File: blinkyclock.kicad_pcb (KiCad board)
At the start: 2 copper layers, 14 parts, among them J1 USB_OTG, J2 RTC, SW1 SW_Push, U1 ATTINY85-20PU

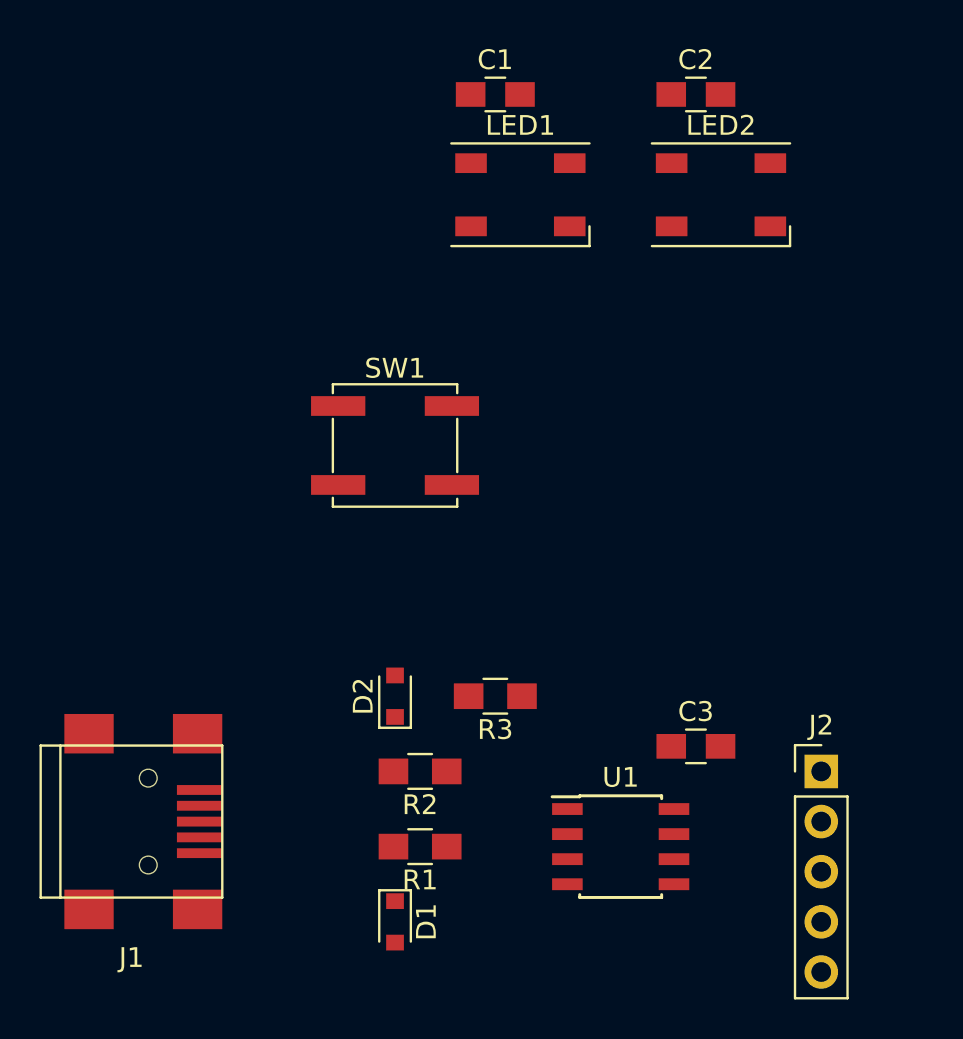
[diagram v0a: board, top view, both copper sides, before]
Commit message: finished layout
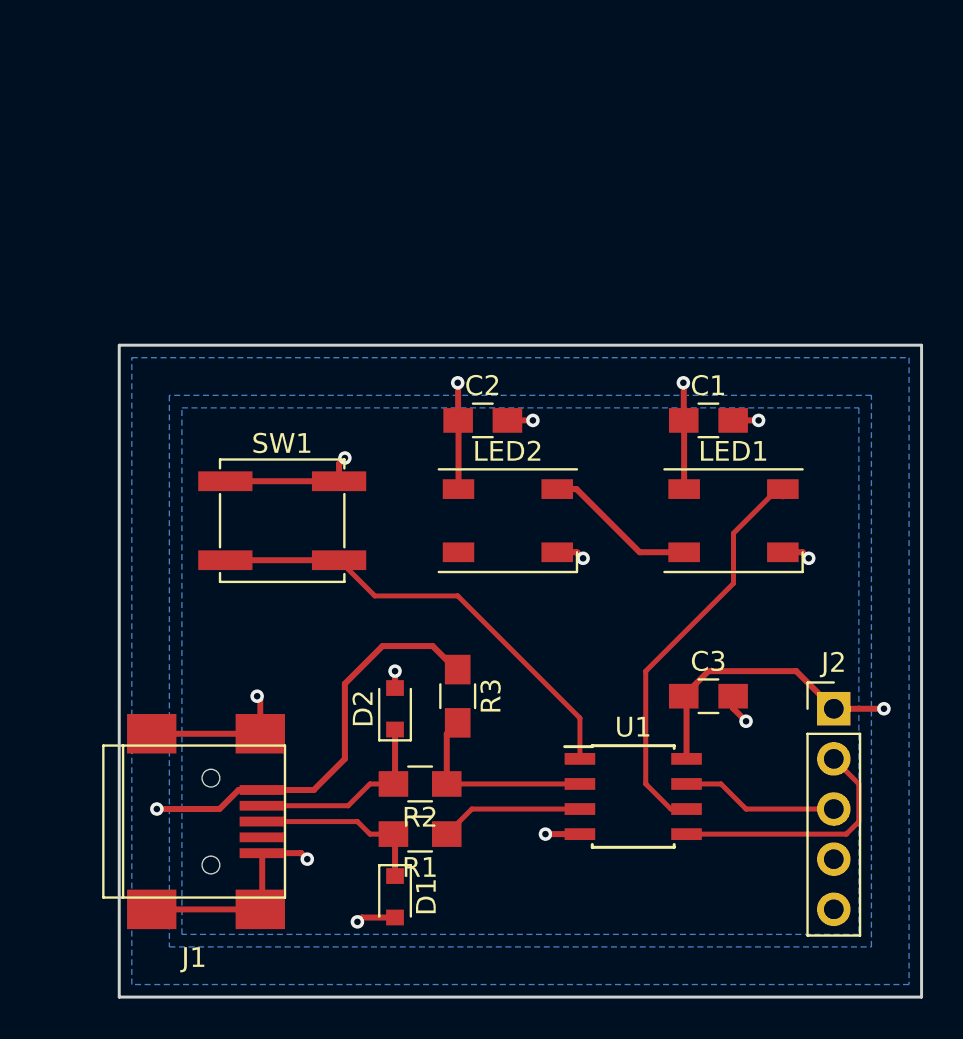
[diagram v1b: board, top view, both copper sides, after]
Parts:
- moved LED2 19.7 mm to (159.4, 104.1)
- moved C1 19.7 mm to (169.5, 99.1)
- moved C2 19.7 mm to (158.1, 99.1)
- moved LED1 19.7 mm to (170.8, 104.1)
- moved SW1 6.87 mm to (148.0, 104.1)
- moved J2 3.24 mm to (175.9, 113.7)
- moved J1 3.18 mm to (144.1, 119.4)
- moved U1 2.62 mm to (165.7, 118.1)
- moved C3 2.62 mm to (169.5, 113.0)
- moved R3 1.91 mm to (156.8, 113.0), turned to 270 degrees
- moved D1 1.27 mm to (153.7, 123.2)
- moved D2 0.64 mm to (153.7, 113.7)
- moved R1 0.64 mm to (154.9, 120.0)
- moved R2 0.63 mm to (154.9, 117.5)
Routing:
- net +5V: track 0.00 -> 46.9 mm, vias 0 -> 4
- net GND: track 0.00 -> 36.9 mm, vias 0 -> 11
- net Net-(SW1-Pad2): track 0.00 -> 23.3 mm
- net Net-(LED1-Pad4): track 0.00 -> 20.9 mm
- net Net-(J2-Pad2): track 0.00 -> 13.3 mm
- net Net-(D2-Pad1): track 0.11 -> 10.6 mm
- net Net-(R2-Pad1): track 0.00 -> 10.1 mm
- net Net-(D1-Pad1): track 0.00 -> 9.07 mm
- net Net-(J2-Pad3): track 0.00 -> 7.99 mm
- net Net-(LED1-Pad2): track 0.00 -> 7.76 mm
- net Net-(R1-Pad1): track 0.00 -> 7.27 mm
- added copper zone on B.Cu, net +5V
- added copper zone on B.Cu, net GND
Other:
- board outline added: 40.6 x 33 mm
- net class Default: clearance 0.2 -> 0.1524; trace_width 0.25 -> 0.1524; via_dia 0.6 -> 0.6858; via_drill 0.4 -> 0.3302
- net class Power added: clearance 0.1524, trace_width 0.3048, via_dia 0.6858, via_drill 0.3302
- rule trace_clearance: 0.2 -> 0.1524
- rule trace_min: 0.2 -> 0.1524
- rule via_min_drill: 0.3 -> 0.3302
- rule via_min_size: 0.4 -> 0.6858
